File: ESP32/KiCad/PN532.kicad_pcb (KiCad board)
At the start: 2 copper layers, 42 x 42 mm, 39 parts, among them J1 Header, J2 SPOX, J3 MiniGrid, SW1 TAMPER, U1 PN532, X1 27.12MHz

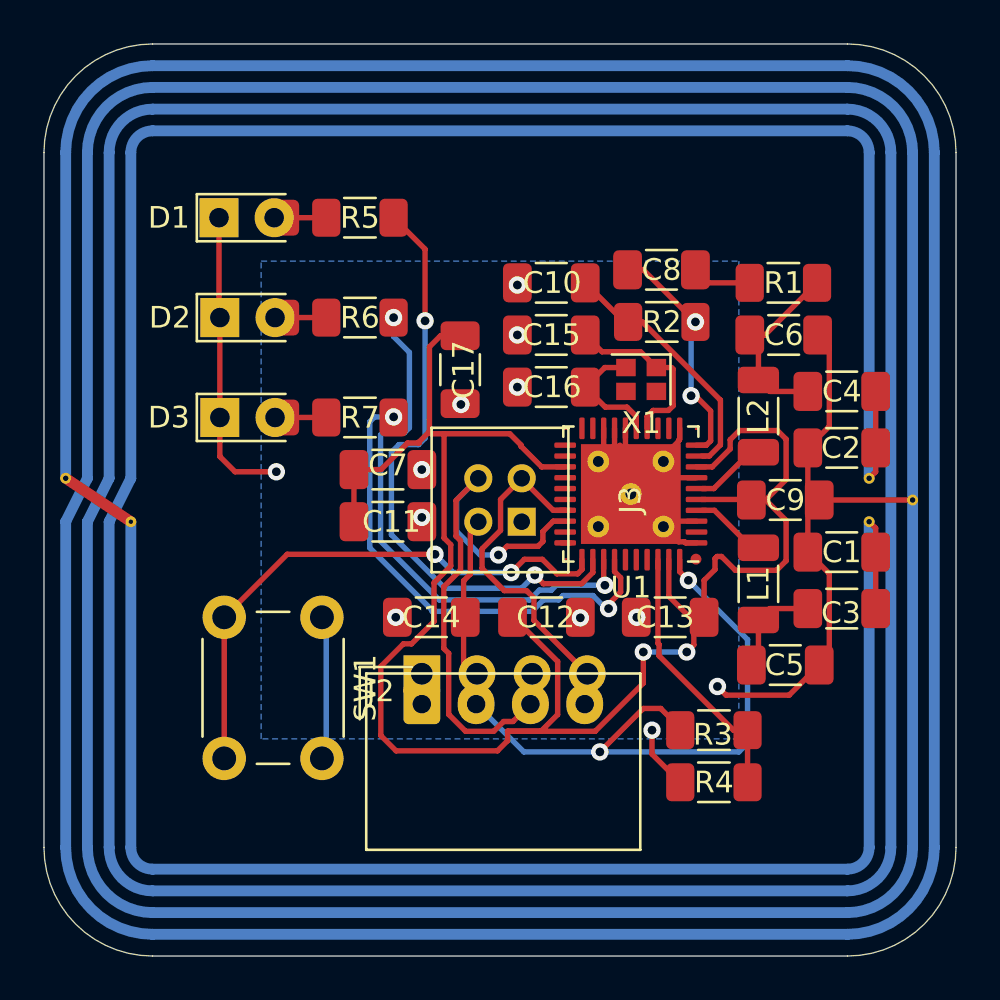
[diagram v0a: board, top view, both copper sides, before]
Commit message: Tracked, and pretty much ready to try it.
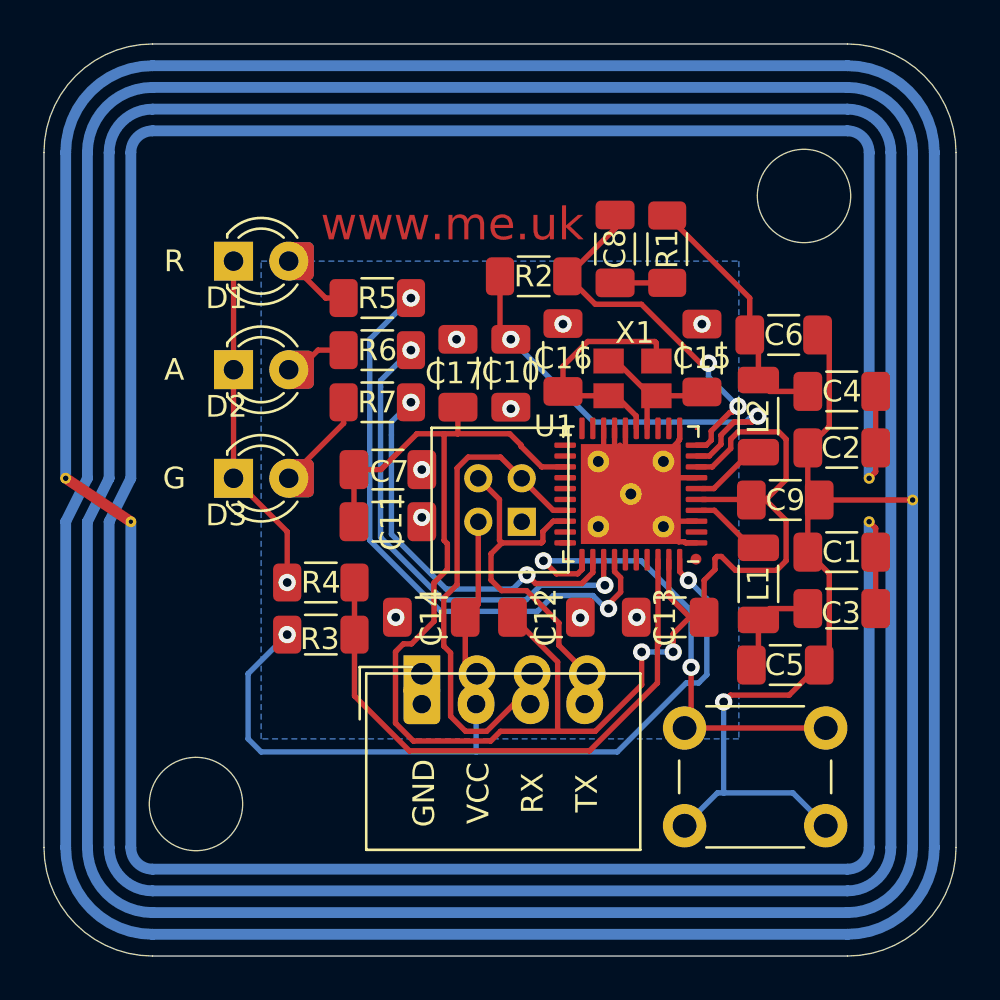
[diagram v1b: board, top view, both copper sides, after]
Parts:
- removed D4: RED, LED_THT:LED_D3.0mm
- removed D5: AMBER, LED_THT:LED_D3.0mm
- removed D6: GREEN, LED_THT:LED_D3.0mm
- added H1: MountingHole, MountingHole:MountingHole_4.3mm_M4, F.Cu at (135.0, 65.0)
- added H2: MountingHole, MountingHole:MountingHole_4.3mm_M4, F.Cu at (107.0, 93.0)
- D1, D2, D3: footprint LED_SMD:LED_1206_3216Metric_Castellated -> RevK:LED_D3.0mm_and_SMD
- X1: value 27.12MHz -> 27.12MHz (Mouser 830053099); footprint Crystal:Crystal_SMD_2016-4Pin_2.0x1.6mm -> RevK:Crystal-3.4x2.7
- moved SW1 25.1 mm to (136.0, 94.0), turned to 180 degrees
- moved R4 20.3 mm to (112.8, 82.8)
- moved R3 18.6 mm to (112.8, 85.2)
- moved C15 7.02 mm to (130.3, 72.5), turned to 90 degrees
- moved R2 6.26 mm to (122.5, 68.7)
- moved R1 5.57 mm to (128.7, 67.5), turned to 90 degrees
- moved C10 4.56 mm to (121.5, 73.2), turned to 270 degrees
- moved R5 3.79 mm to (115.3, 69.7)
- moved D3 2.84 mm to (110.0, 78.0)
- moved D2 2.45 mm to (110.0, 73.0)
- moved C8 2.34 mm to (126.3, 67.4), turned to 270 degrees
- moved D1 2.06 mm to (110.0, 68.0)
- moved R6 1.70 mm to (115.3, 72.1)
- moved C16 1.46 mm to (123.9, 72.4), turned to 90 degrees
- moved R7 1.06 mm to (115.3, 74.5)
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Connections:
- J3 pad 3: Net-(J1-Pad4) -> Net-(J1-Pad3)
- J3 pad 4: Net-(J1-Pad3) -> Net-(J1-Pad4)
- U1 pad 27: Net-(J1-Pad4) -> Net-(J1-Pad3)
- U1 pad 28: Net-(J1-Pad3) -> Net-(J1-Pad4)
- U1 pad 32: Net-(R5-Pad1) -> Net-(R7-Pad1)
- U1 pad 34: Net-(R7-Pad1) -> Net-(R5-Pad1)
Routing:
- net Net-(R3-Pad1): track 12.3 -> 27.5 mm
- net +3V3: track 87.1 -> 78.3 mm
- net Net-(C10-Pad1): track 11.6 -> 20.0 mm, vias 0 -> 2
- net +5V: track 38.7 -> 45.3 mm
- net Net-(C8-Pad1): track 10.9 -> 17.3 mm
- net Net-(C16-Pad1): track 5.71 -> 11.2 mm
- net Net-(R7-Pad1): track 22.4 -> 18.0 mm
- net GND: track 81.4 -> 85.5 mm, vias 12 -> 11
- net Net-(J1-Pad3): track 27.4 -> 24.3 mm, vias 1 -> 0
- net Net-(C4-Pad2): track 8.83 -> 11.8 mm
- net Net-(SW1-Pad2): track 25.6 -> 22.8 mm
- net Net-(D3-Pad2): track 2.05 -> 4.55 mm
- net Net-(R6-Pad1): track 24.7 -> 22.2 mm
- net Net-(C15-Pad1): track 8.34 -> 6.71 mm
- net Net-(D1-Pad2): track 2.05 -> 3.23 mm
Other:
- board text added: "A"
- board text added: "G"
- board text added: "GND"
- board text added: "R"
- board text added: "RX"
- board text added: "TX"
- board text added: "VCC"
- board text added: "www.me.uk"
